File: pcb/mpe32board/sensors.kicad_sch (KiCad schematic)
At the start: 93 parts, among them U4 TCA9548ARGER, U5 TCA9548ARGER, U6 TCA9548ARGER, U7 TCA9548ARGER, U8 TCA9548ARGER

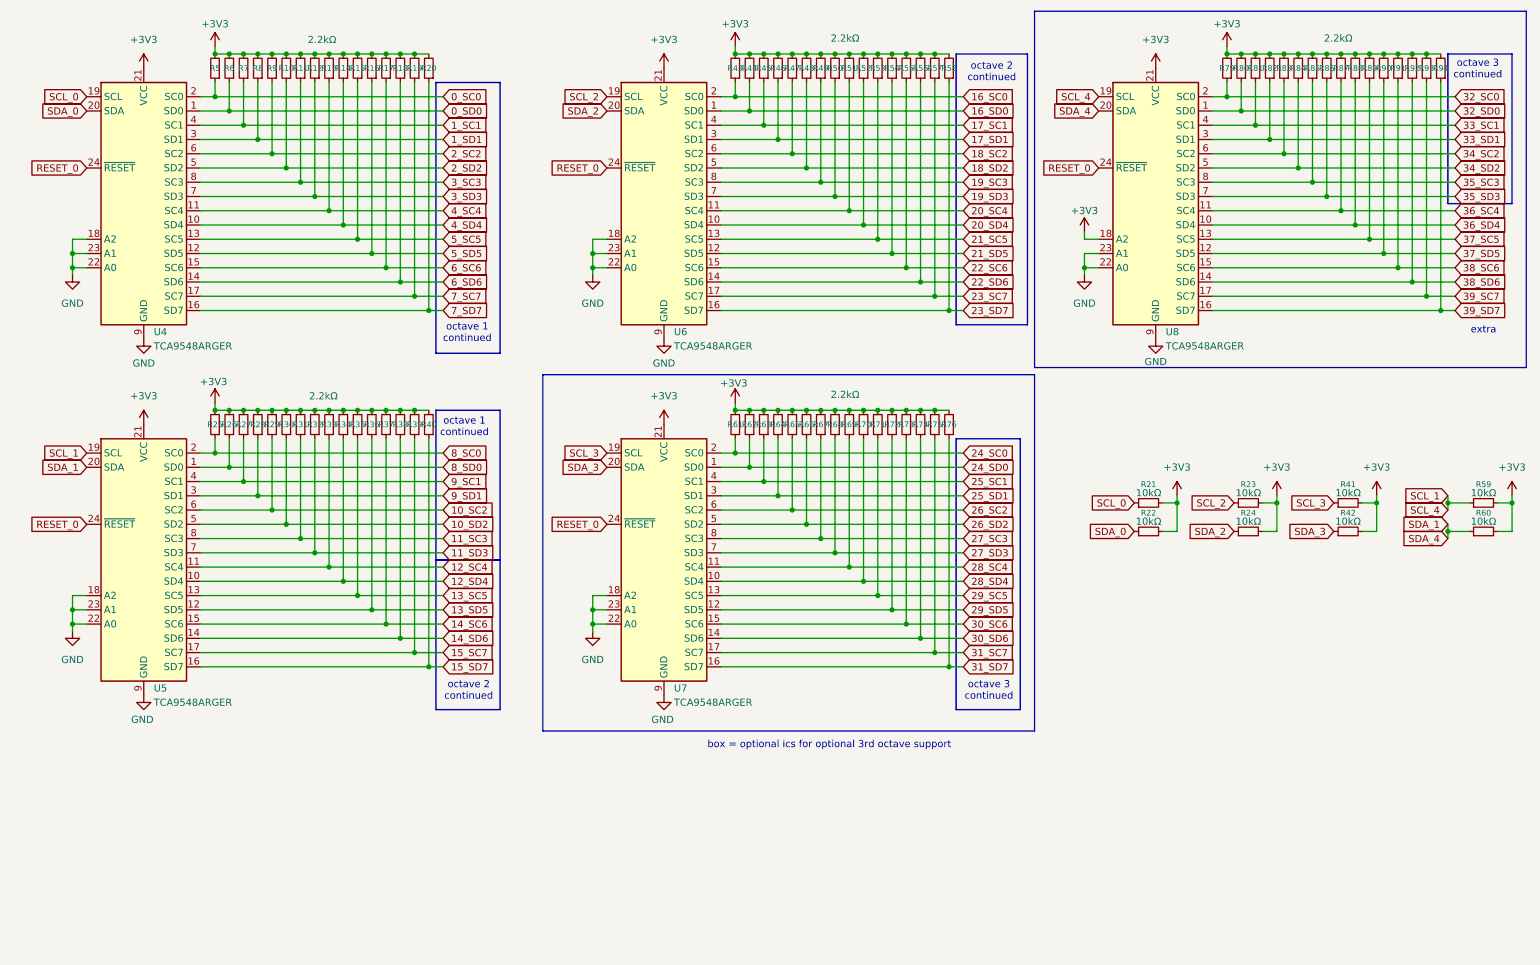
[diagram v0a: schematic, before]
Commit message: codec
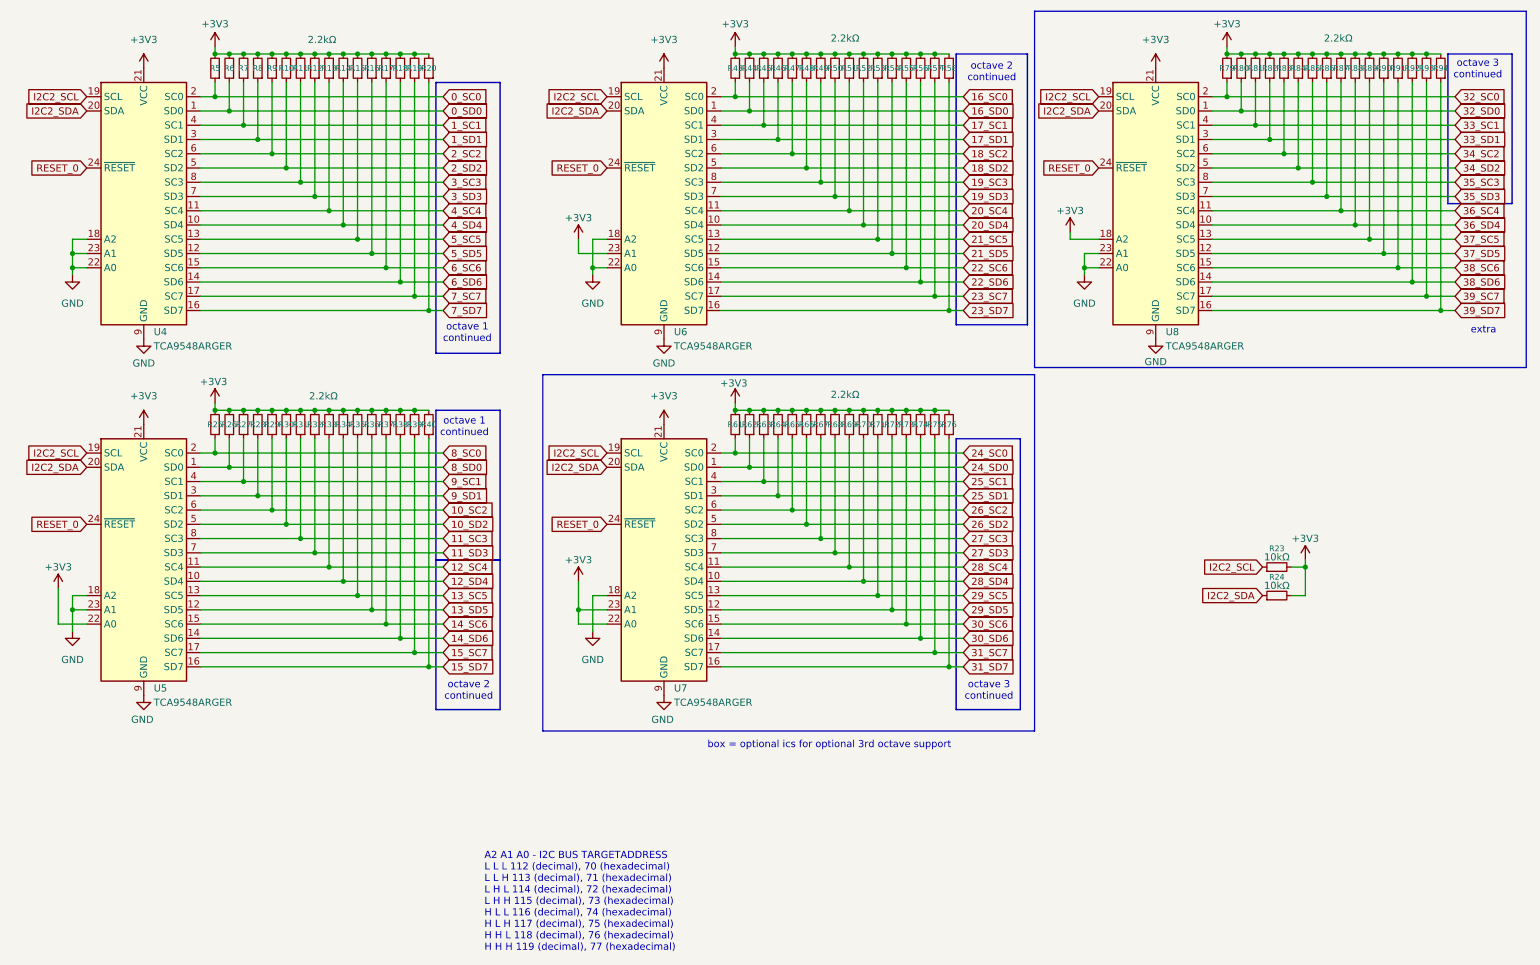
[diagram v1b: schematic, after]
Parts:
- removed R21, R22, R41, R42, R59, R60: 10kΩ, symbol Device:R_Small
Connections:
- net SCL_1 is gone; now on net I2C2_SCL: U5.19 (SCL), U8.19 (SCL)
- net SCL_2 is gone; now on net I2C2_SCL: R23.1, U6.19 (SCL)
- net SCL_3 is gone; now on net I2C2_SCL: U7.19 (SCL)
- net SDA_1 is gone; now on net I2C2_SDA: U5.20 (SDA), U8.20 (SDA)
- net SDA_2 is gone; now on net I2C2_SDA: R24.1, U6.20 (SDA)
- net SDA_3 is gone; now on net I2C2_SDA: U7.20 (SDA)
- net +3V3: now also U5.22 (A0), U6.23 (A1), U7.22 (A0), U7.23 (A1)
- net GND: no longer U5.22 (A0), U6.23 (A1), U7.22 (A0), U7.23 (A1)
- net SCL_0 renamed I2C2_SCL
- net SDA_0 renamed I2C2_SDA
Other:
- note added: "A2 A1 A0 - I2C BUS TARGETADDRESS L L L 112 (decimal), 70 (hexadecimal) L L H 113 (decimal), 71 (hexadecimal) L H L 114 (decimal), 72 (hexadecimal) L H H 115 (decimal), 73 (hexadecimal) H L L 116 (decimal), 74 (hexadecimal) H L H 117 (decimal), 75 (hexadecimal) H H L 118 (decimal), 76 (hexadecimal) H H H 119 (decimal), 77 (hexadecimal)"
- moved on the sheet: R23, R24

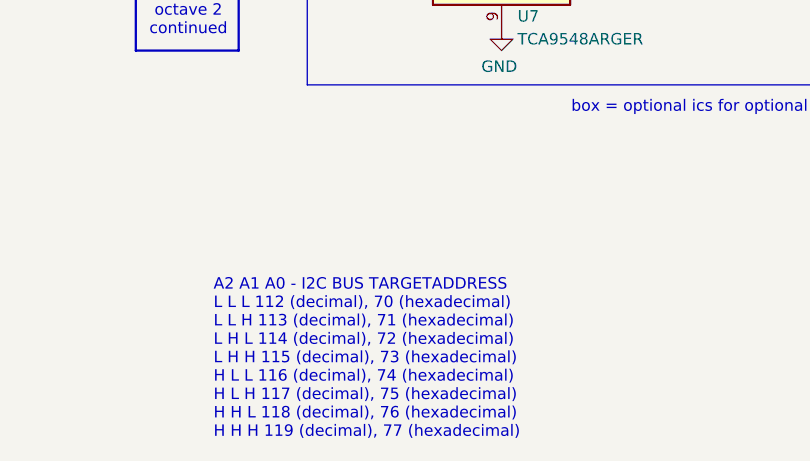
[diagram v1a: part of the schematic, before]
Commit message: layout stuff
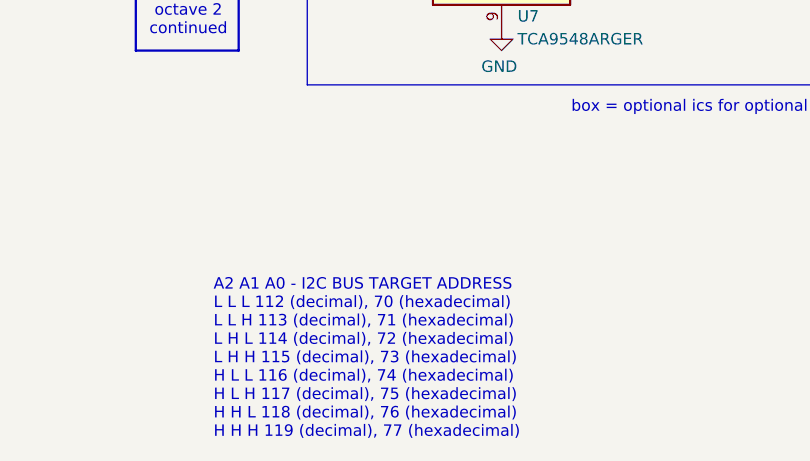
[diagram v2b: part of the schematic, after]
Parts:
- R10, R11, R12, R13, R14, R15, R16, R17, R18, R19, R20, R23, R24, R25, R26, R27, R28, R29, R30, R31, R32, R33, R34, R35, R36, R37, R38, R39, R40, R43, R44, R45, R46, R47, R48, R49, R5, R50, R51, R52, R53, R54, R55, R56, R57, R58, R6, R61, R62, R63, R64, R65, R66, R67, R68, R69, R7, R70, R71, R72, R73, R74, R75, R76, R79, R8, R80, R81, R82, R83, R84, R85, R86, R87, R88, R89, R9, R90, R91, R92, R93, R94: footprint (none) -> Resistor_SMD:R_0603_1608Metric
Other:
- note added: "A2 A1 A0 - I2C BUS TARGET ADDRESS L L L 112 (decimal), 70 (hexadecimal) L L H 113 (decimal), 71 (hexadecimal) L H L 114 (decimal), 72 (hexadecimal) L H H 115 (decimal), 73 (hexadecimal) H L L 116 (decimal), 74 (hexadecimal) H L H 117 (decimal), 75 (hexadecimal) H H L 118 (decimal), 76 (hexadecimal) H H H 119 (decimal), 77 (hexadecimal)"
- note removed: "A2 A1 A0 - I2C BUS TARGETADDRESS L L L 112 (decimal), 70 (hexadecimal) L L H 113 (decimal), 71 (hexadecimal) L H L 114 (decimal), 72 (hexadecimal) L H H 115 (decimal), 73 (hexadecimal) H L L 116 (decimal), 74 (hexadecimal) H L H 117 (decimal), 75 (hexadecimal) H H L 118 (decimal), 76 (hexadecimal) H H H 119 (decimal), 77 (hexadecimal)"

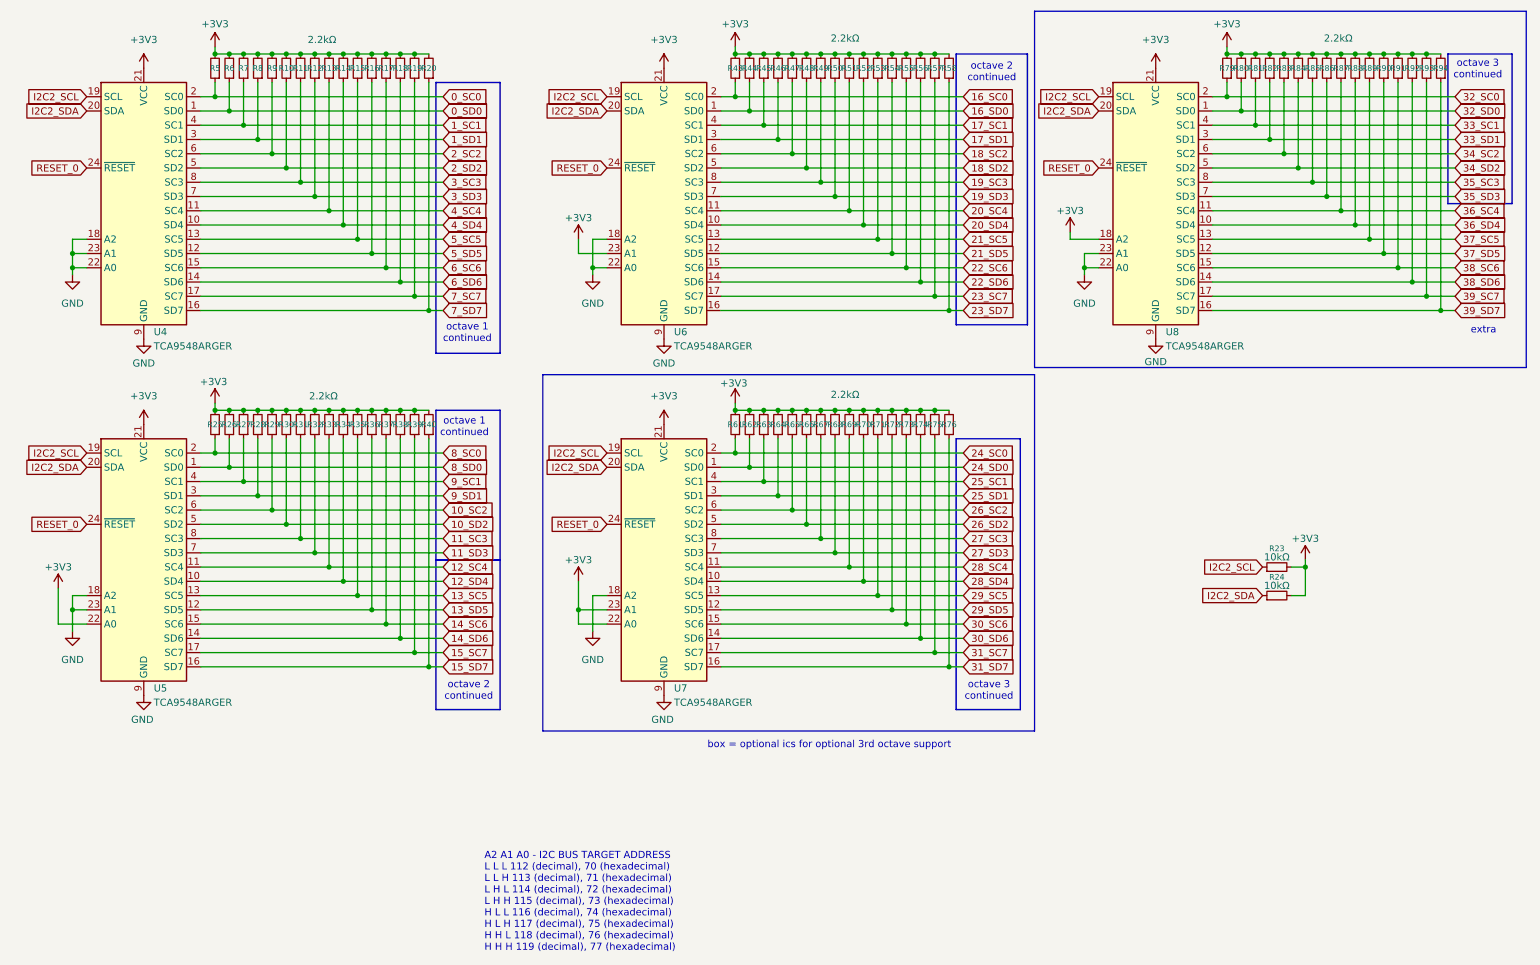
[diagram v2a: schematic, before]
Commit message: board layout stuff
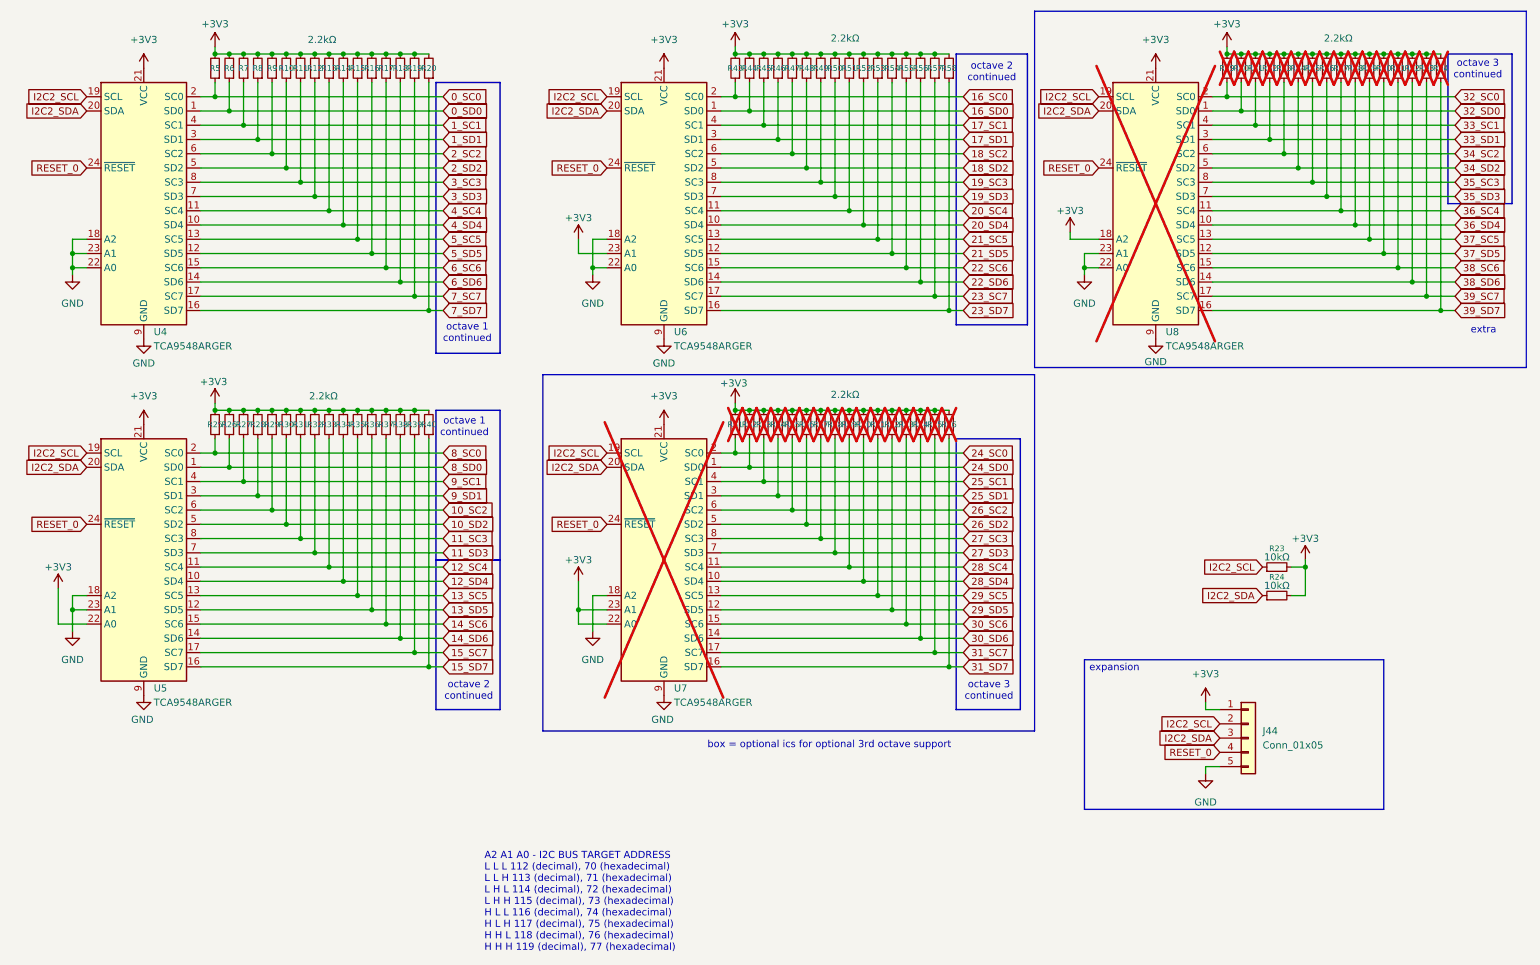
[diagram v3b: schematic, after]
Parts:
- added J44: Conn_01x05, Connector_Molex:Molex_SL_171971-0005_1x05_P2.54mm_Vertical, symbol Connector_Generic:Conn_01x05
- R61, R62, R63, R64, R65, R66, R67, R68, R69, R70, R71, R72, R73, R74, R75, R76, R79, R80, R81, R82, R83, R84, R85, R86, R87, R88, R89, R90, R91, R92, R93, R94, U7, U8: now not fitted; now left out of the parts list
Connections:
- net +3V3: now also J44.1 (Pin_1)
- net GND: now also J44.5 (Pin_5)
- net I2C2_SCL: now also J44.2 (Pin_2)
- net I2C2_SDA: now also J44.3 (Pin_3)
- net RESET_0: now also J44.4 (Pin_4)
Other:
- note added: "expansion"

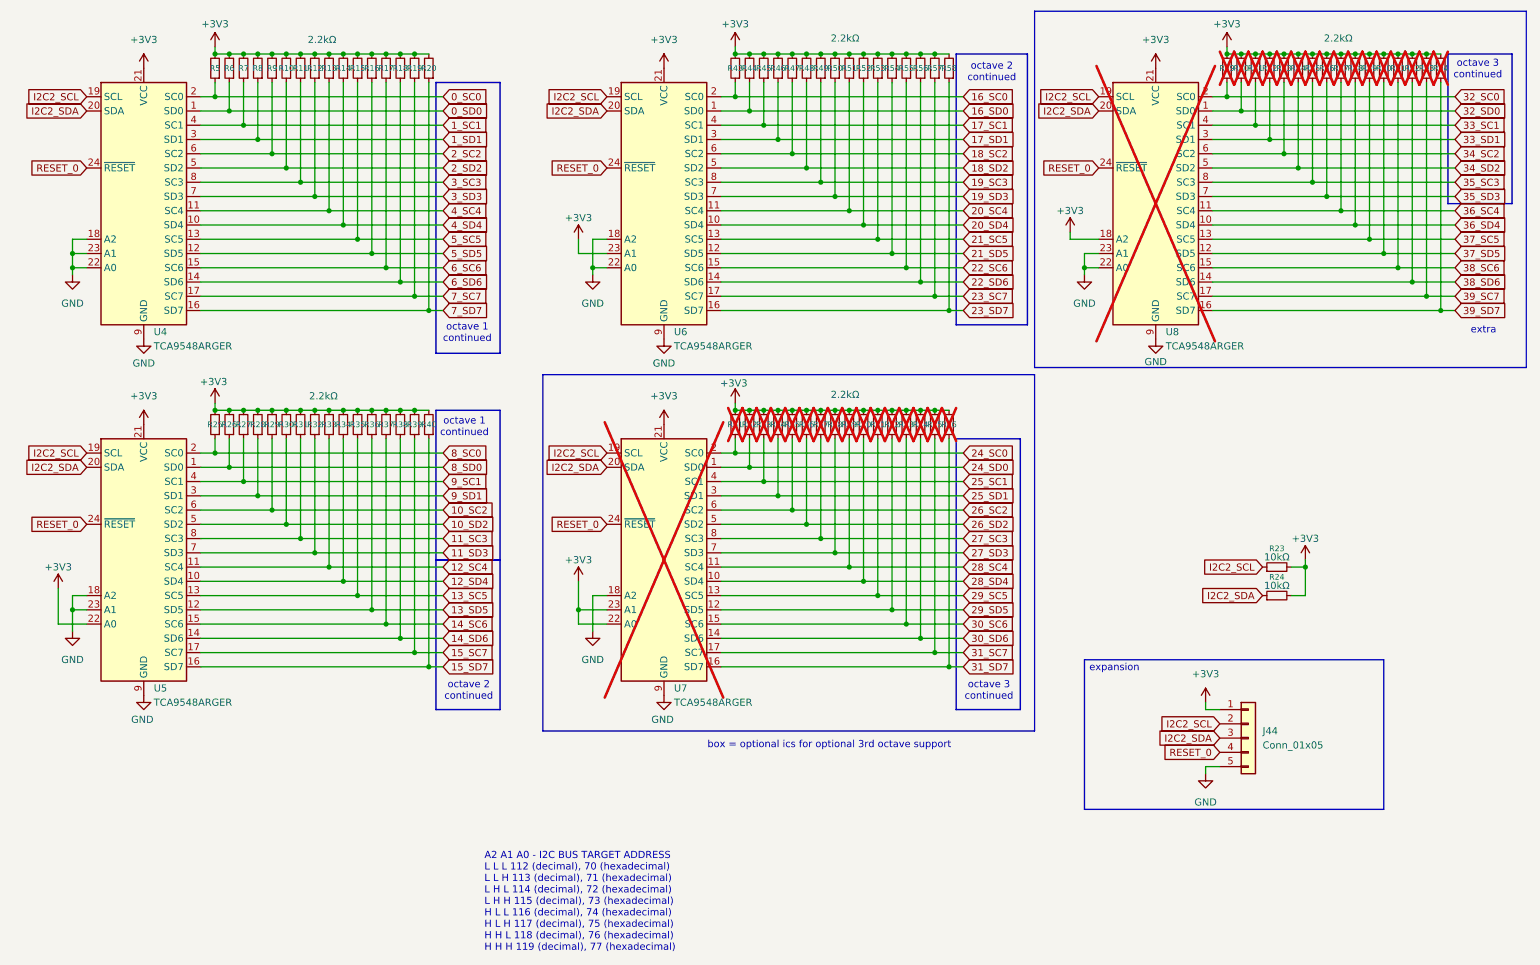
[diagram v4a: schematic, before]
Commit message: routed ram
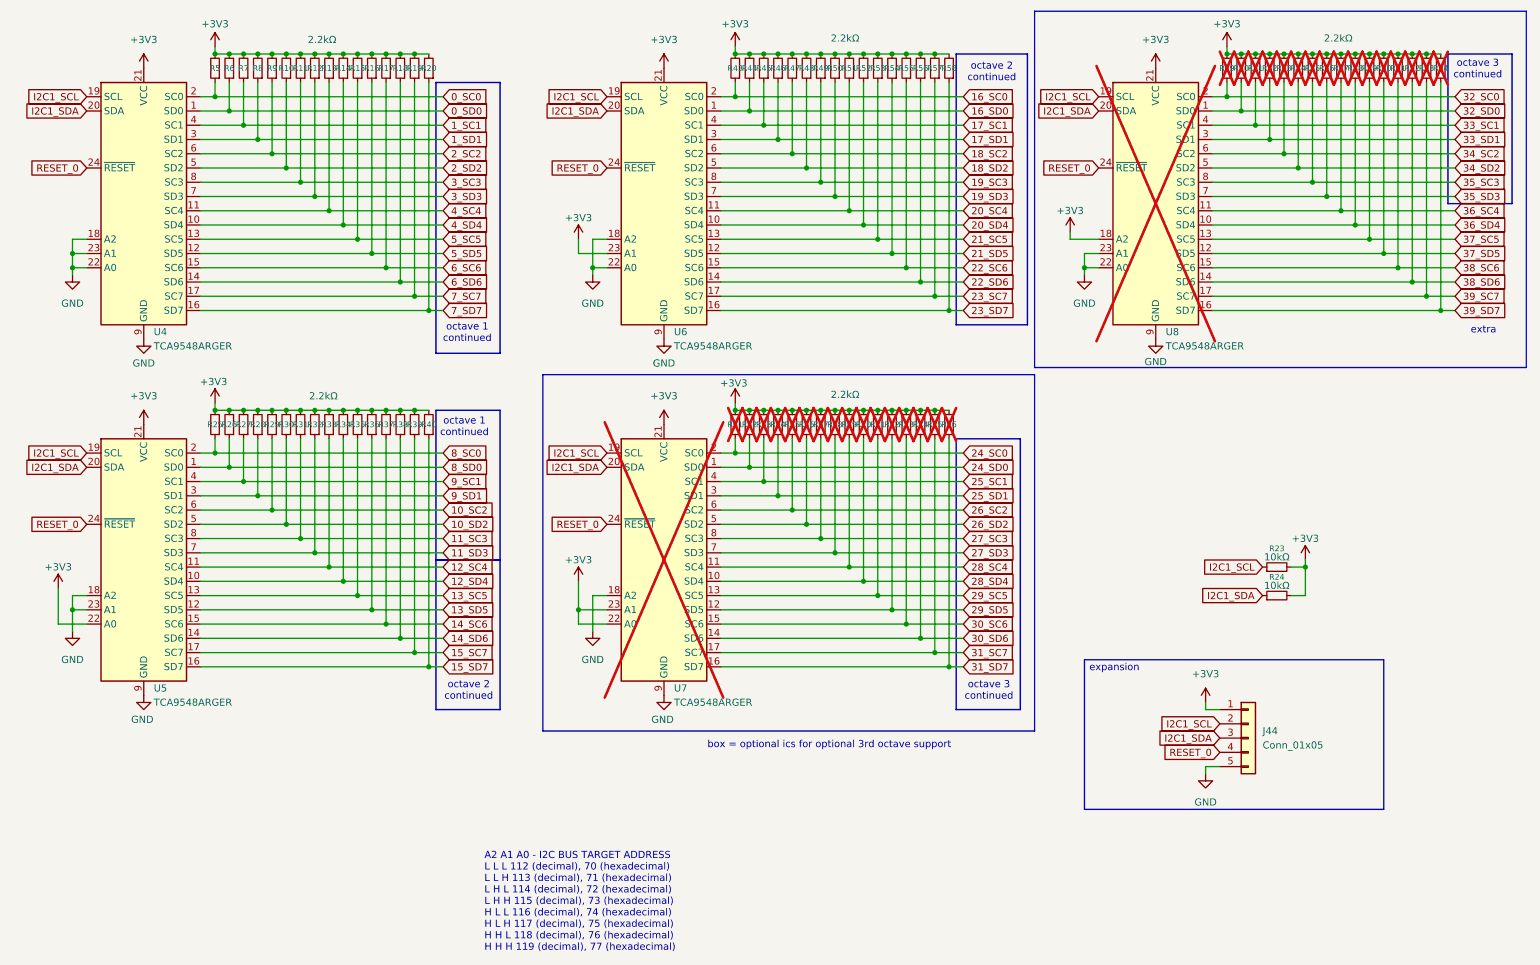
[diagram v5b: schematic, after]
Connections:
- net I2C2_SCL renamed I2C1_SCL
- net I2C2_SDA renamed I2C1_SDA
